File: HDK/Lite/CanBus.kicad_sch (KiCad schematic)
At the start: 10 parts, among them J201 TERM, U201 SN65HVD230, U202 MCP2518FD, Y201 40MHz

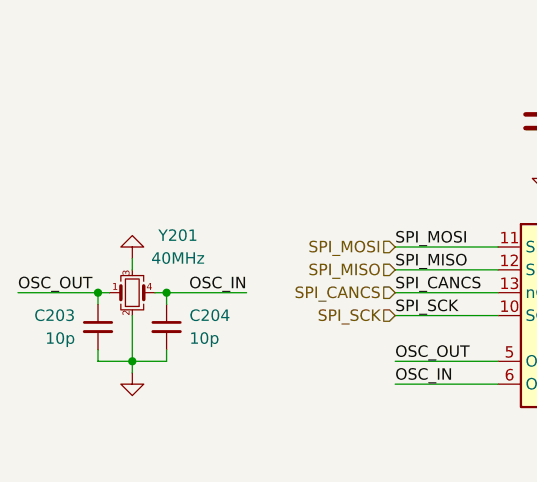
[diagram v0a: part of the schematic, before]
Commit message: updated 1 Job, WIP
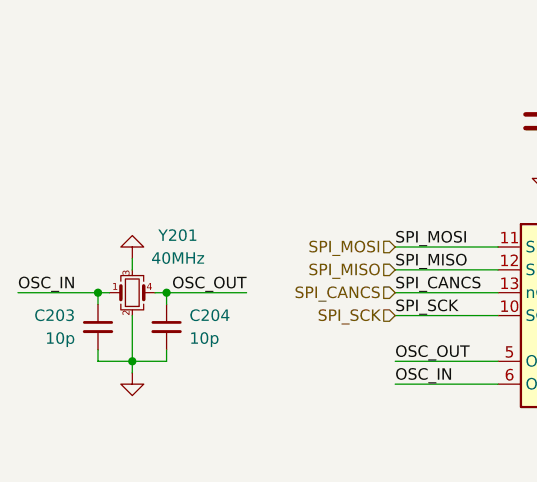
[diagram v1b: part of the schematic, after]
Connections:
- net OSC_IN: now also C203.1, Y201.1; no longer C204.1, Y201.4
- net OSC_OUT: now also C204.1, Y201.4; no longer C203.1, Y201.1
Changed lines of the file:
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@@
     (effects (font (size 1.27 1.27)) (justify left bottom))
   )
-  (label "OSC_OUT" (at 68.58 87.63 0) (fields_autoplaced)
-    (effects (font (size 1.27 1.27)) (justify left bottom))
+  (label "OSC_OUT" (at 93.98 87.63 180) (fields_autoplaced)
+    (effects (font (size 1.27 1.27)) (justify right bottom))
   )
   (label "OSC_IN" (at 110.49 97.79 0) (fields_autoplaced)
     (effects (font (size 1.27 1.27)) (justify left bottom))
   )
-  (label "OSC_IN" (at 93.98 87.63 180) (fields_autoplaced)
-    (effects (font (size 1.27 1.27)) (justify right bottom))
+  (label "OSC_IN" (at 68.58 87.63 0) (fields_autoplaced)
+    (effects (font (size 1.27 1.27)) (justify left bottom))
   )
   (label "SPI_CANCS" (at 110.49 87.63 0) (fields_autoplaced)
